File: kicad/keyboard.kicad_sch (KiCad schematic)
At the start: 8 parts, among them J1 Conn_01x07_Male, J2 Conn_01x07_Male, SW1 SW_Push, U1 Arduino_pro_Micro

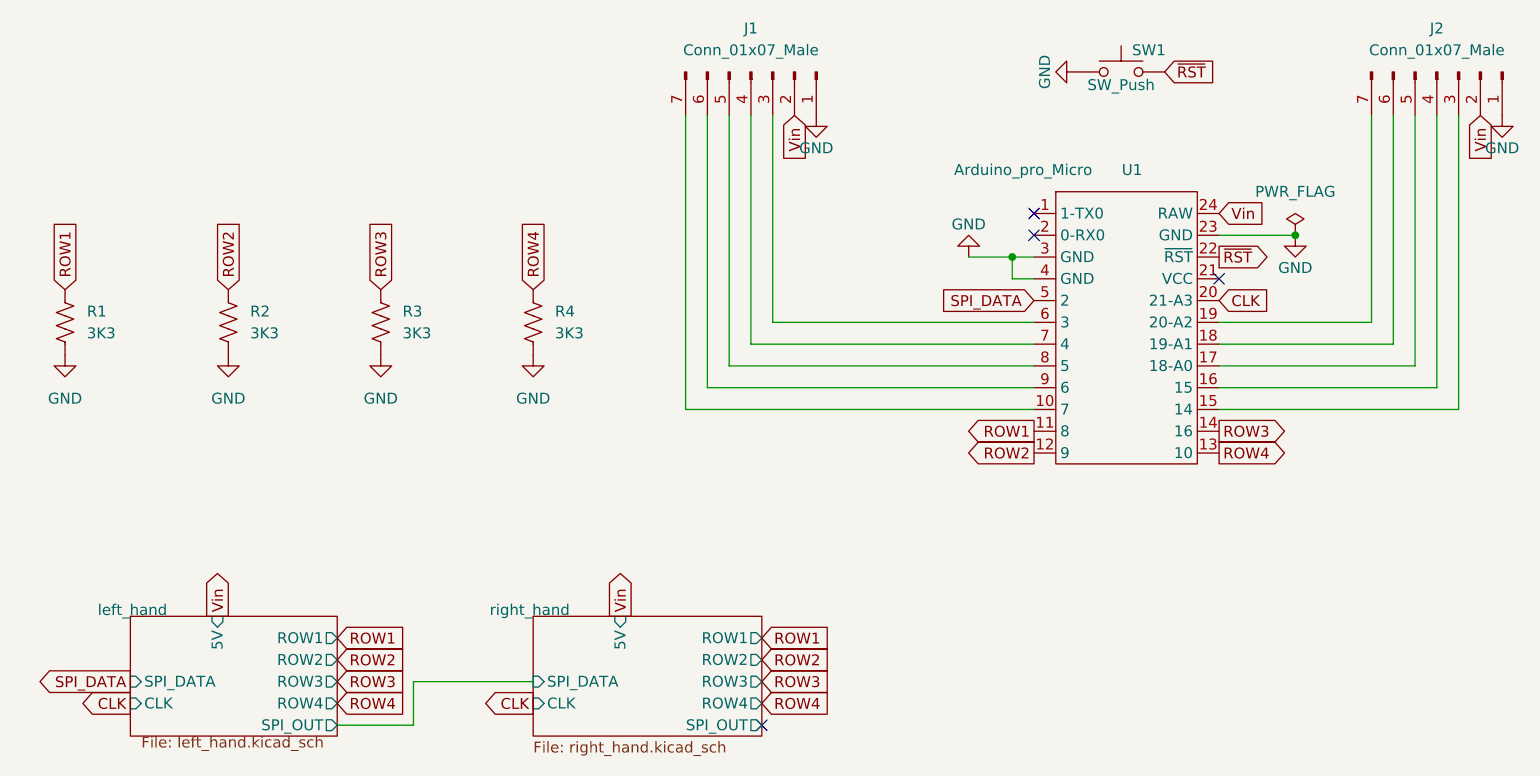
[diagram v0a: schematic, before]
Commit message: Update PCB
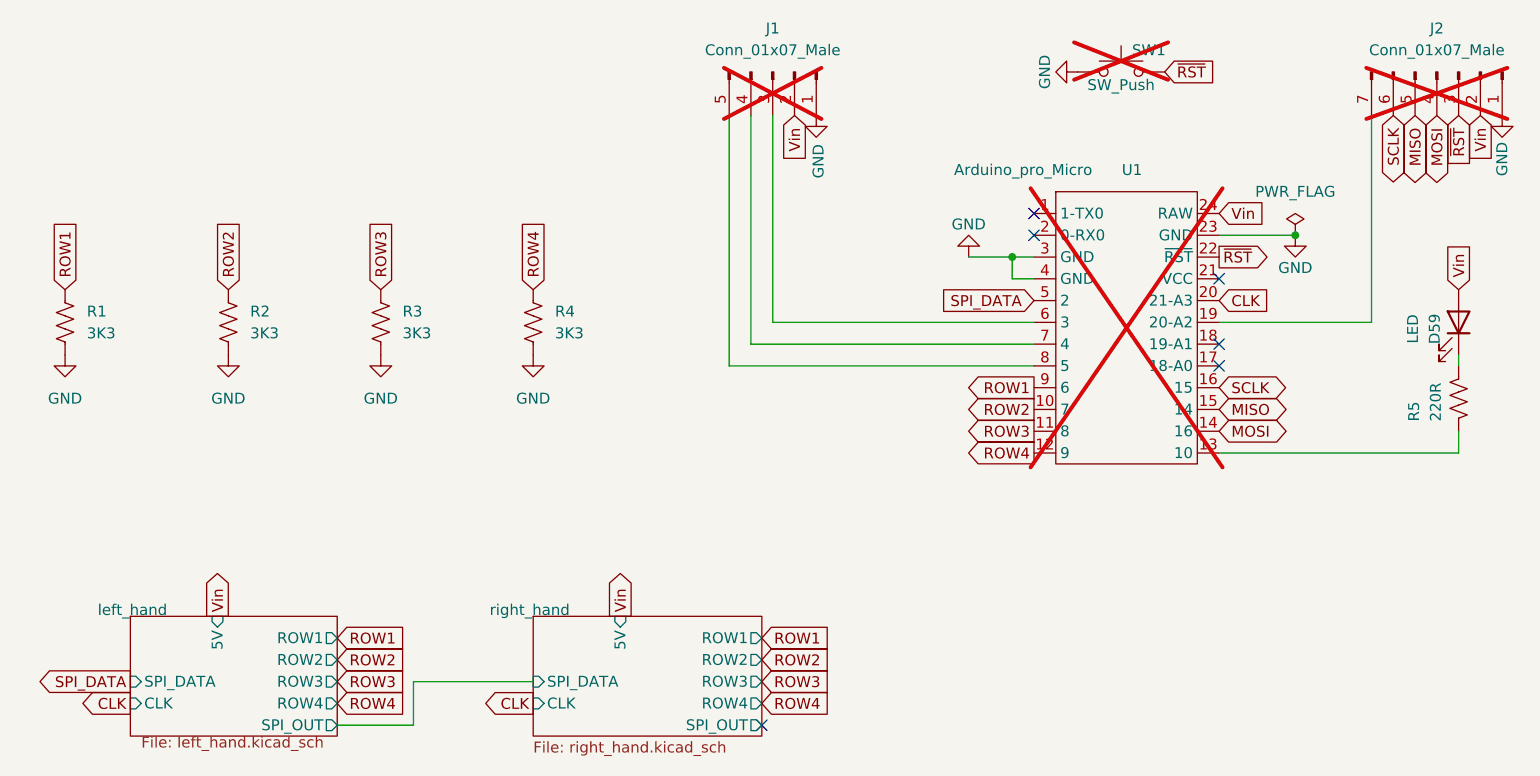
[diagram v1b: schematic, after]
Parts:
- added D59: LED, LED_SMD:LED_0805_2012Metric, symbol Device:LED
- added R5: 220R, Resistor_SMD:R_0603_1608Metric, symbol Device:R_US
- J1: footprint Keyboard:PinHeader_01x07 -> Connector_PinHeader_2.54mm:PinHeader_1x05_P2.54mm_Vertical; symbol Connector:Conn_01x07_Pin -> Connector:Conn_01x05_Pin; now not fitted
- J2, SW1, U1: now not fitted
- R1, R2, R3, R4: footprint Resistor_THT:R_Axial_DIN0207_L6.3mm_D2.5mm_P7.62mm_Horizontal -> Resistor_SMD:R_0603_1608Metric; LCSC (none) -> C22978
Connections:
- net ROW1: now also U1.9 (6); no longer U1.11 (8)
- net ROW2: now also U1.10 (7); no longer U1.12 (9)
- net ROW3: now also U1.11 (8); no longer U1.14 (16)
- net ROW4: now also U1.12 (9); no longer U1.13 (10)
- net Vin: now also D59.2 (A)
- net ~{RST}: now also J2.3 (Pin_3)
- net MISO: now reaches U1.15 (14)
- net MISO: now also J2.5 (Pin_5); no longer J2.3 (Pin_3)
- net MOSI: now reaches J2.4 (Pin_4)
- net MOSI: now also U1.14 (16); no longer U1.16 (15)
- net at U1.17 (18-A0): no longer J2.5 (Pin_5)
- net at U1.18 (19-A1): no longer J2.6 (Pin_6)
- new net: R5.1, U1.13 (10)
- new net: D59.1 (K), R5.2
- new net SCLK: J2.6 (Pin_6), U1.16 (15)
- no-connect marks 4 -> 6
